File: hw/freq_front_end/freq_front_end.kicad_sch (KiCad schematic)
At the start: 7 parts, among them J1 Conn_Coaxial, U1 OPA310SxDBV, U2 74LVC1G17, U3 SN74LV161APWR, U4 HMC363, U5 BFP196

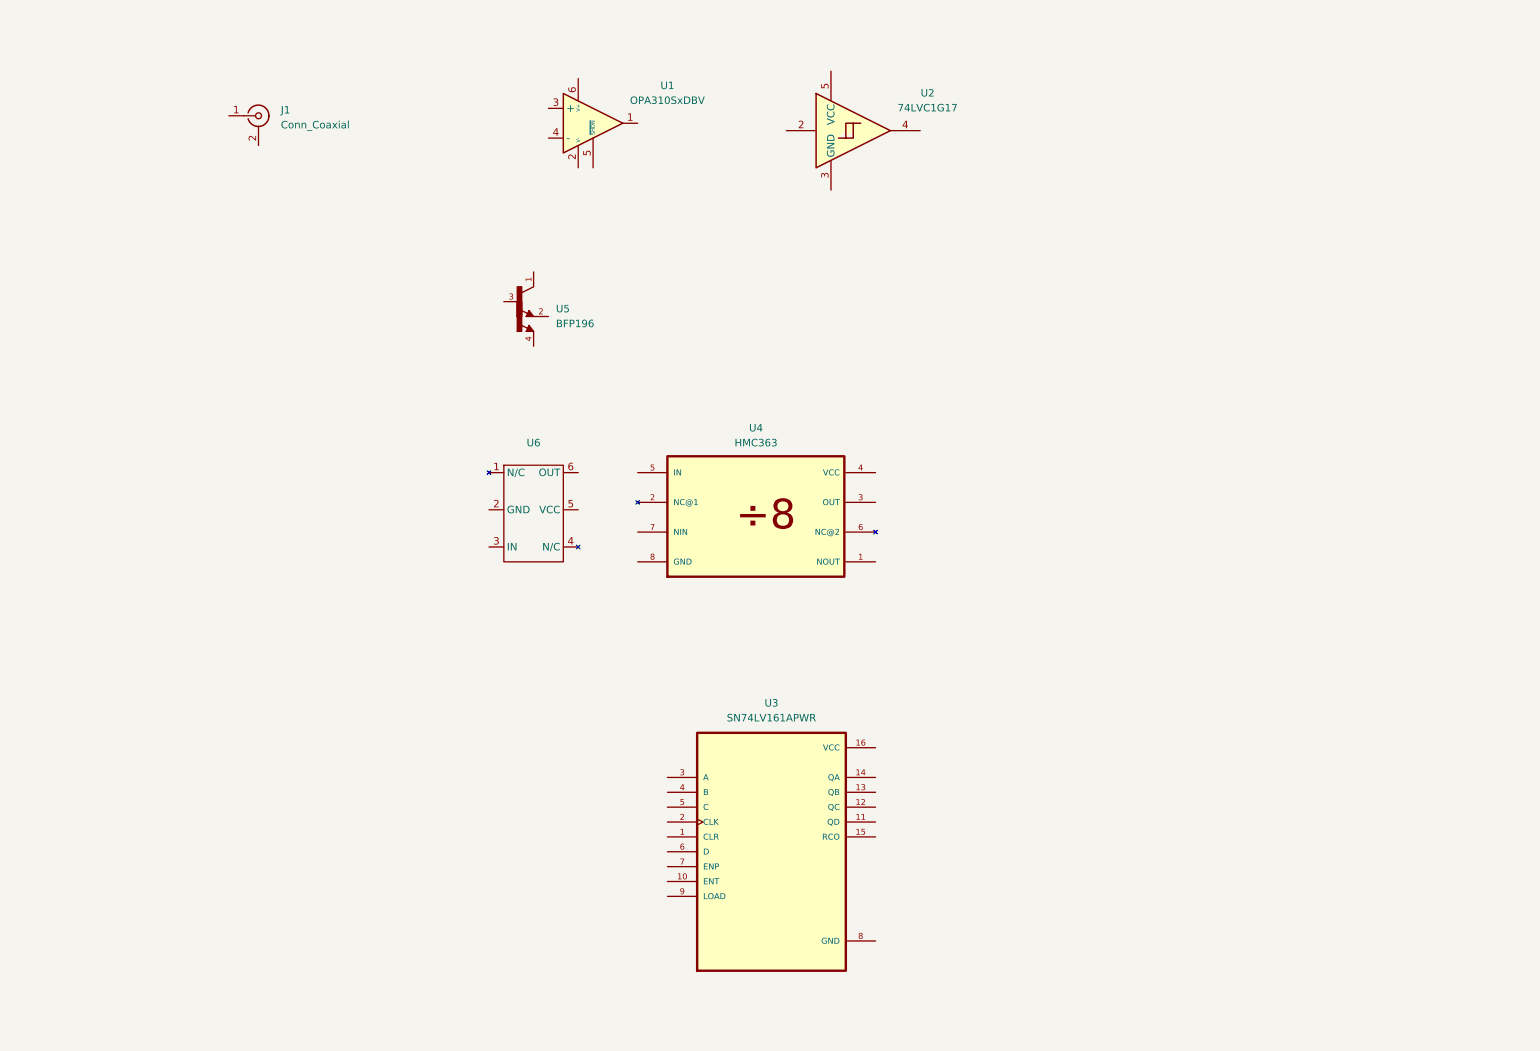
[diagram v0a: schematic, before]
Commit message: 108 - schematic wip
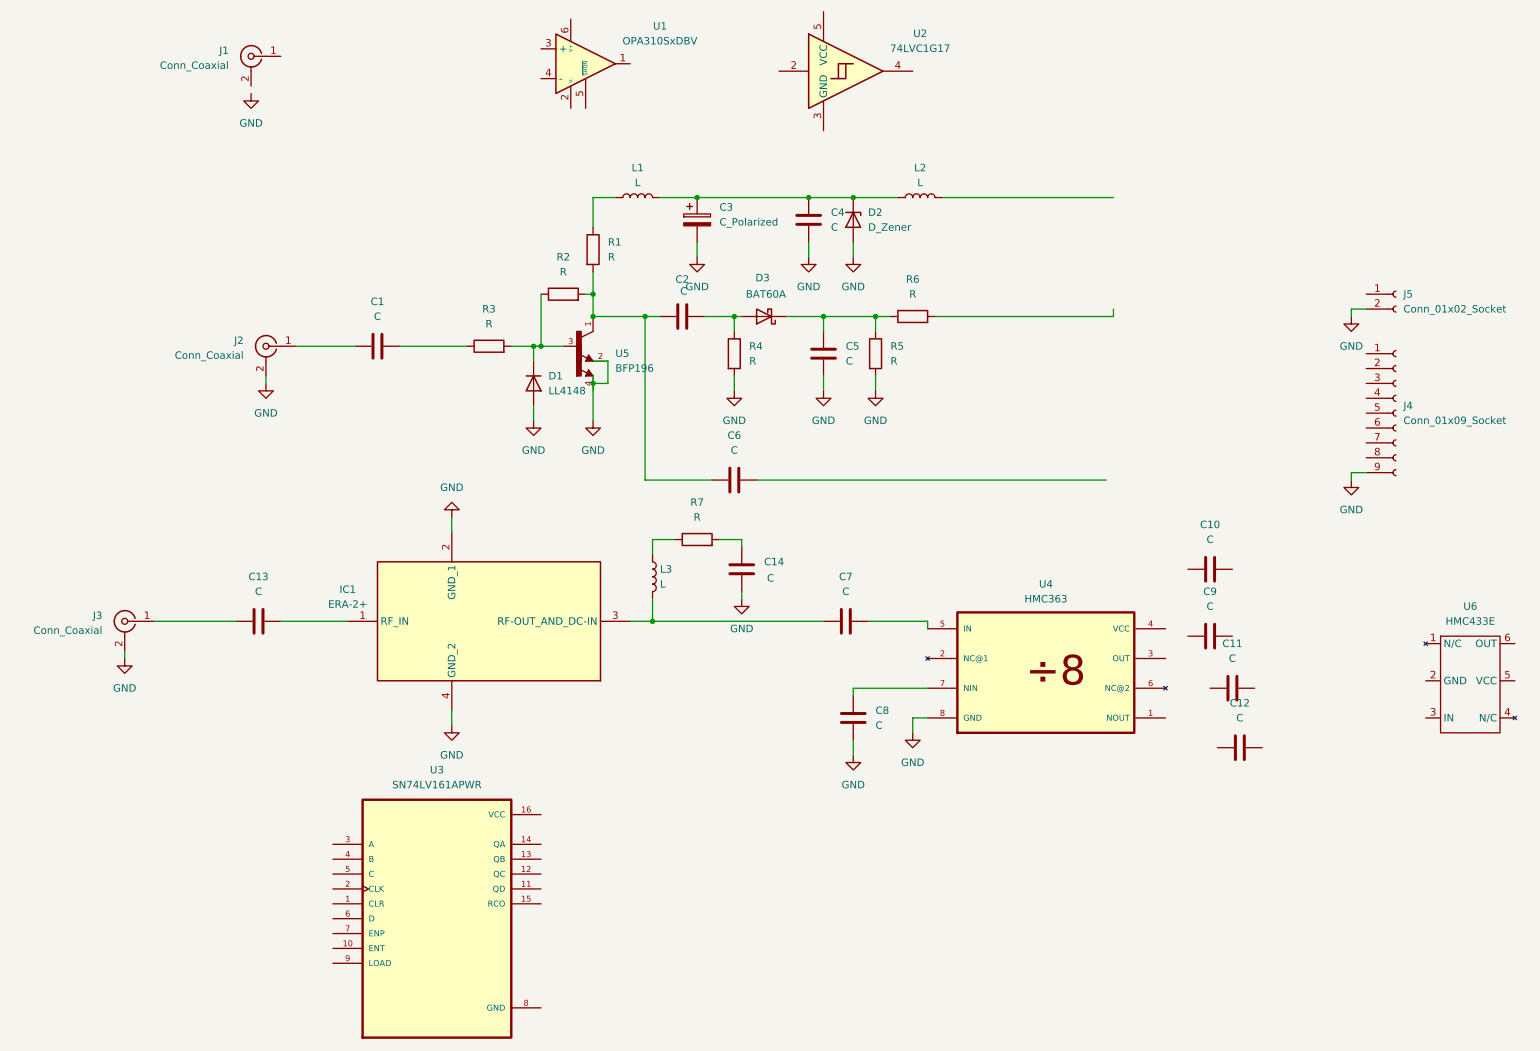
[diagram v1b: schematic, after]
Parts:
- added C1, C2: C, Capacitor_SMD:C_1206_3216Metric, symbol Device:C
- added C10, C11, C12, C13, C14, C4, C5, C6, C7, C8, C9: C, symbol Device:C
- added C3: C_Polarized, symbol Device:C_Polarized
- added D1: LL4148, Diode_SMD:D_MiniMELF, symbol Diode:LL4148
- added D2: D_Zener, symbol Device:D_Zener
- added D3: BAT60A, Diode_SMD:D_SOD-323, symbol Diode:BAT60A
- added IC1: ERA-2+, ERA2, symbol f4bjh_library:ERA-2+
- added J2, J3: Conn_Coaxial, symbol Connector:Conn_Coaxial
- added J4: Conn_01x09_Socket, symbol Connector:Conn_01x09_Socket
- added J5: Conn_01x02_Socket, symbol Connector:Conn_01x02_Socket
- added L1, L2, L3: L, symbol Device:L
- added R1, R2, R3, R4, R7: R, Resistor_SMD:R_1206_3216Metric, symbol Device:R
- added R5, R6: R, symbol Device:R
- U6: value ~ -> HMC433E
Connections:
- net at U4.5 (IN): now also C7.2
- net at U4.7 (NIN): now also C8.2
- net GND: now reaches U4.8 (GND)
- net GND: now also U5.2, U5.4, C14.1, C3.2, C4.2, C5.2, C8.1, D1.2 (A), D2.2 (A), IC1.2 (GND_1), IC1.4 (GND_2), J2.2 (Ext), J3.2 (Ext), J4.9 (Pin_9), J5.2 (Pin_2), R4.2, R5.2
- net at U5.1: now also C2.1, C6.1, R1.2, R2.2
- net at U5.3: now also D1.1 (K), R2.1, R3.2
- new net: L1.1, R1.1
- new net: C3.1, C4.1, D2.1 (K), L1.2, L2.1
- new net: C5.1, D3.1 (K), R5.1, R6.1
- new net: C7.1, IC1.3 (RF-OUT_AND_DC-IN), L3.2
- new net: C2.2, D3.2 (A), R4.1
- new net: L3.1, R7.1
- new net: C14.2, R7.2
- new net: C1.2, R3.1
- new net: C13.2, IC1.1 (RF_IN)
- new net: C1.1, J2.1 (In)
- new net: C13.1, J3.1 (In)
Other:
- moved on the sheet: J1, U1, U2, U3, U4, U5, U6
